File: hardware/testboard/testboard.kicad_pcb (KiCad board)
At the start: 2 copper layers, 175 x 140 mm, 22 parts, among them J1 Reset, P1 Conn_01x06, P2 Conn_01x06, U1 68LC040, U10 SN74ALVC164245, U11 ICE40HX4K-TQ144, U13 SST26VF023BA, U14 SN74ALVC164245, U15 SN74ALVC164245, U2 MAX232, U3 MAX232, U4 68681, U6 IS61C5128AS-25TLI, U7 IS61C5128AS-25TLI, U8 NB3N502, X1 ASE-33MHz, X2 33MHz, X3 33MHz

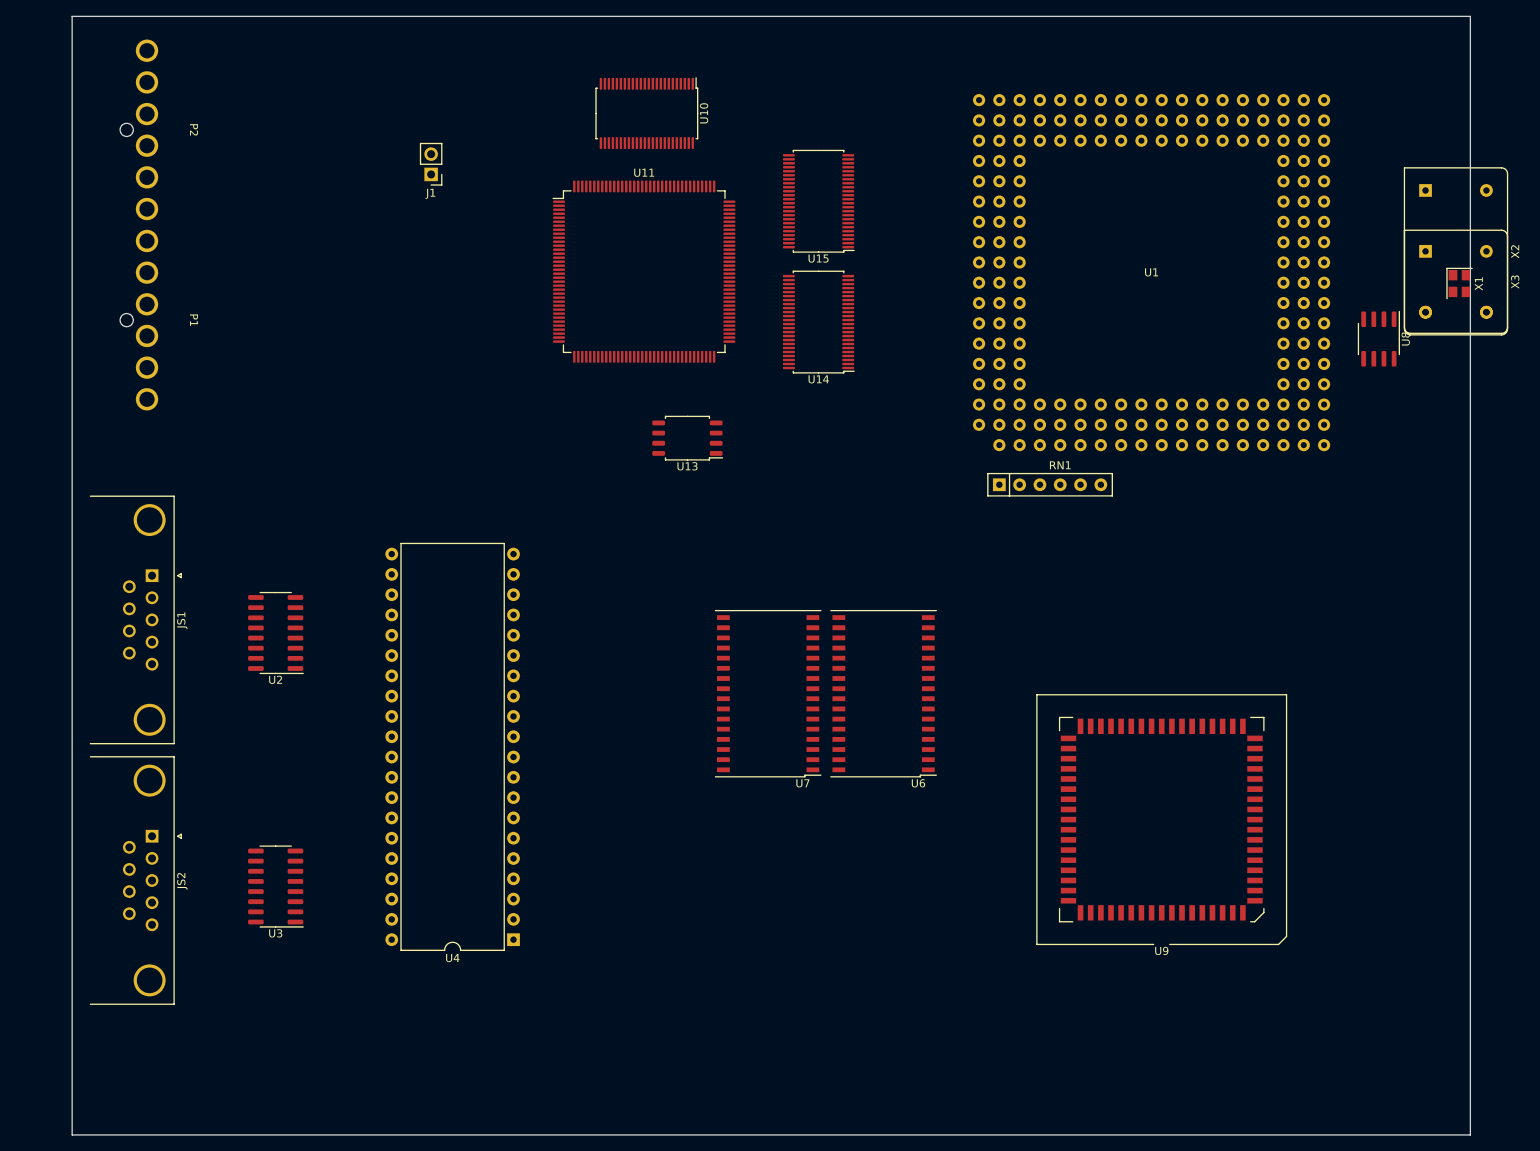
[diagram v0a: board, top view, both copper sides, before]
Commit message: simpleboard nearly complete
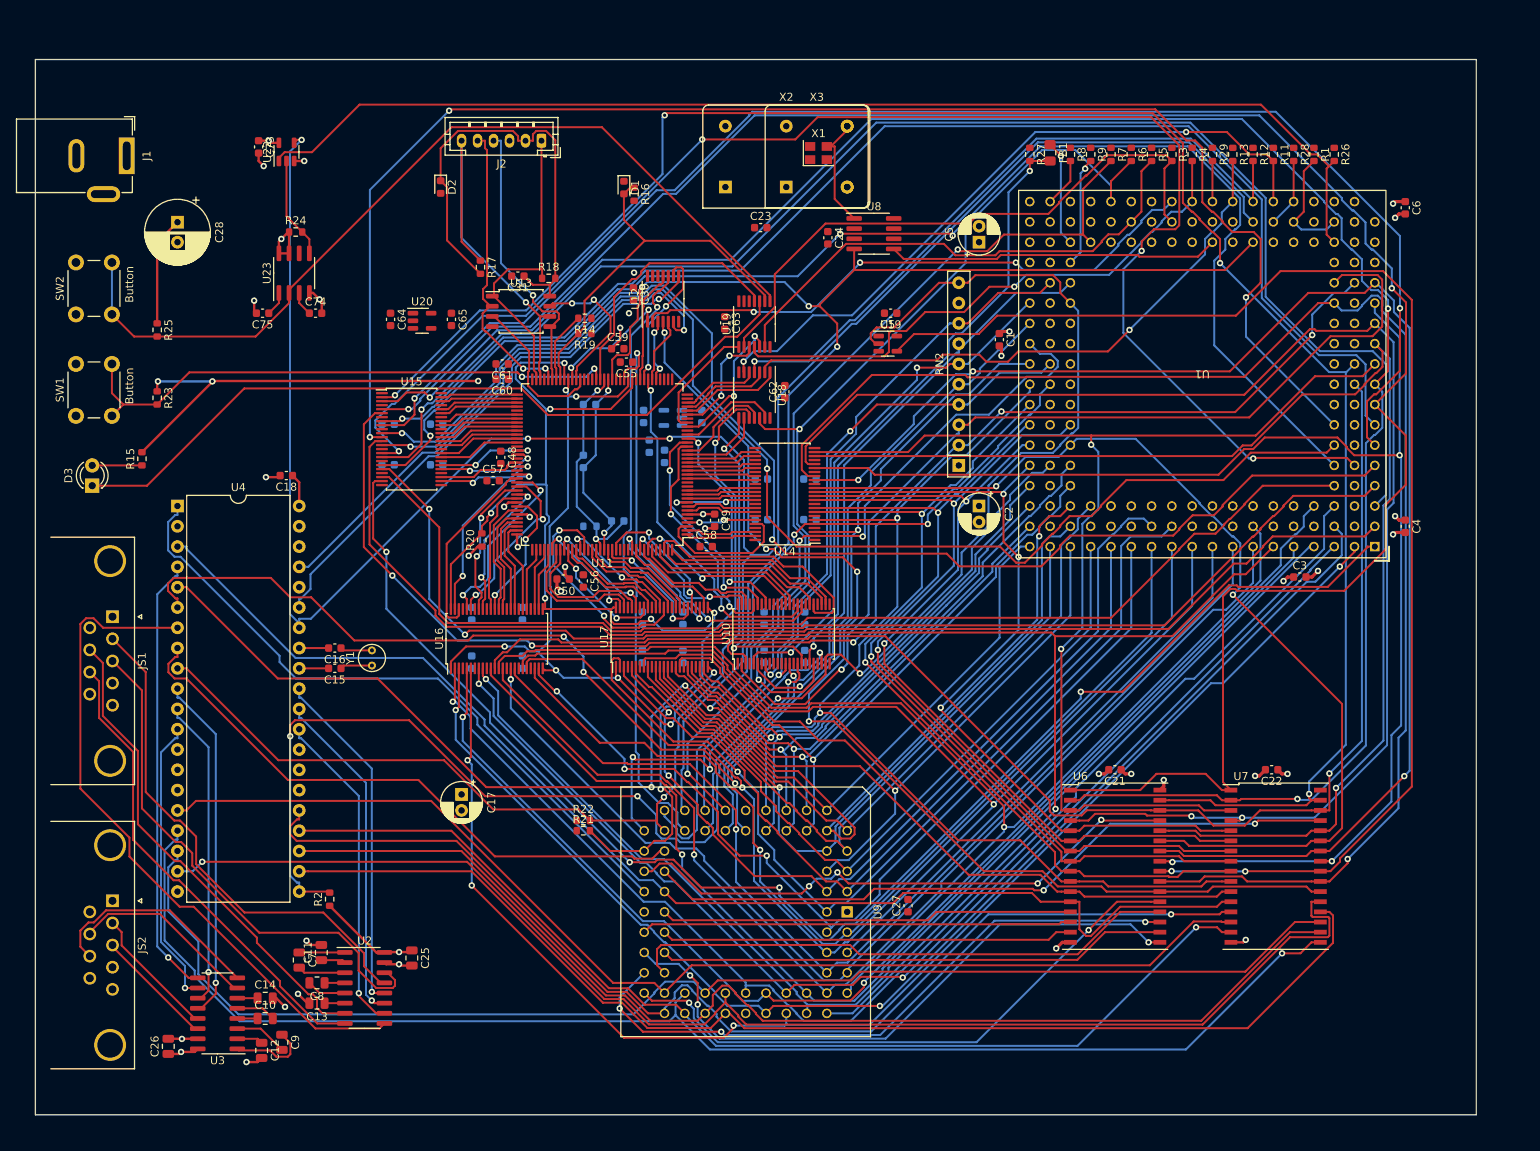
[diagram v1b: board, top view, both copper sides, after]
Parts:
- removed P1, P2: Conn_01x06, 68040:15-48-0106
- removed RN1: 4.7k, Resistor_THT:R_Array_SIP6
- added C1: 0.22uF, Capacitor_SMD:C_0603_1608Metric, F.Cu at (146.1, 60.5)
- added C10: 1uF, Capacitor_SMD:C_0805_2012Metric, F.Cu at (54.2, 145.4)
- added C11: 1uF, Capacitor_SMD:C_0805_2012Metric, F.Cu at (61.2, 137.2)
- added C12: 1uF, Capacitor_SMD:C_0805_2012Metric, F.Cu at (53.7, 149.4)
- added C13: 1uF, Capacitor_SMD:C_0805_2012Metric, F.Cu at (60.6, 143.5)
- added C14: 1uF, Capacitor_SMD:C_0805_2012Metric, F.Cu at (54.2, 142.9)
- added C15: 15pF, Capacitor_SMD:C_0603_1608Metric, F.Cu at (62.9, 101.6)
- added C16: 15pF, Capacitor_SMD:C_0603_1608Metric, F.Cu at (62.9, 99.1)
- added C17: C_Polarized_Small_US, Capacitor_THT:CP_Radial_D5.0mm_P2.00mm, F.Cu at (78.7, 117.4)
- added C18: 100nF, Capacitor_SMD:C_0603_1608Metric, F.Cu at (56.8, 77.5)
- added C19: 100nF, Capacitor_SMD:C_0603_1608Metric, F.Cu at (132.4, 57.1)
- added C2: 22uF, Capacitor_THT:CP_Radial_D5.0mm_P2.00mm, F.Cu at (143.5, 81.3)
- added C21: 100nF, Capacitor_SMD:C_0603_1608Metric, F.Cu at (160.5, 114.3)
- added C22: 100nF, Capacitor_SMD:C_0603_1608Metric, F.Cu at (180.1, 114.3)
- added C23: 100nF, Capacitor_SMD:C_0603_1608Metric, F.Cu at (116.2, 46.4)
- added C24: 100nF, Capacitor_SMD:C_0603_1608Metric, F.Cu at (124.6, 47.7)
- added C25: 1uF, Capacitor_SMD:C_0805_2012Metric, F.Cu at (72.5, 137.9)
- added C26: 1uF, Capacitor_SMD:C_0805_2012Metric, F.Cu at (42.0, 148.9)
- added C27: 100nF, Capacitor_SMD:C_0603_1608Metric, F.Cu at (134.6, 131.3)
- added C28: 220uF, Capacitor_THT:CP_Radial_D8.0mm_P2.50mm, F.Cu at (43.2, 45.8)
- added C3: 220pF, Capacitor_SMD:C_0603_1608Metric, F.Cu at (183.7, 90.2)
- added C30: 100nF, Capacitor_SMD:C_0603_1608Metric, F.Cu at (100.2, 54.8)
- added C31: 100nF, Capacitor_SMD:C_0603_1608Metric, F.Cu at (85.8, 52.5)
- added C32: 100nF, Capacitor_SMD:C_0603_1608Metric, B.Cu at (122.3, 83.0)
- added C33: 100nF, Capacitor_SMD:C_0603_1608Metric, B.Cu at (122.3, 77.9)
- added C34: 100nF, Capacitor_SMD:C_0603_1608Metric, B.Cu at (116.3, 83.0)
- added C35: 100nF, Capacitor_SMD:C_0603_1608Metric, B.Cu at (116.3, 77.9)
- added C36: 100nF, Capacitor_SMD:C_0603_1608Metric, B.Cu at (75.6, 71.0)
- added C37: 100nF, Capacitor_SMD:C_0603_1608Metric, B.Cu at (75.6, 76.1)
- added C38: 100nF, Capacitor_SMD:C_0603_1608Metric, B.Cu at (69.5, 76.1)
- added C39: 100nF, Capacitor_SMD:C_0603_1608Metric, B.Cu at (69.5, 71.0)
- added C4: 0.22uF, Capacitor_SMD:C_0603_1608Metric, F.Cu at (196.8, 83.8)
- added C40: 100nF, Capacitor_SMD:C_0603_1608Metric, B.Cu at (101.4, 100.1)
- added C41: 100nF, Capacitor_SMD:C_0603_1608Metric, B.Cu at (80.0, 94.8)
- added C42: 100nF, Capacitor_SMD:C_0603_1608Metric, B.Cu at (86.4, 94.8)
- added C43: 100nF, Capacitor_SMD:C_0603_1608Metric, B.Cu at (106.4, 100.1)
- added C44: 100nF, Capacitor_SMD:C_0603_1608Metric, B.Cu at (101.4, 95.3)
- added C45: 100nF, Capacitor_SMD:C_0603_1608Metric, B.Cu at (80.0, 100.8)
- added C46: 100nF, Capacitor_SMD:C_0603_1608Metric, B.Cu at (106.4, 95.3)
- added C47: 100nF, Capacitor_SMD:C_0603_1608Metric, B.Cu at (86.4, 100.8)
- added C48: 100nF, Capacitor_SMD:C_0603_1608Metric, F.Cu at (83.6, 75.2)
- added C49: 100nF, Capacitor_SMD:C_0603_1608Metric, F.Cu at (110.4, 83.1)
- added C5: 22uF, Capacitor_THT:CP_Radial_D5.0mm_P2.00mm, F.Cu at (143.5, 48.3)
- added C50: 100nF, Capacitor_SMD:C_0603_1608Metric, F.Cu at (91.5, 90.4)
- added C51: 100nF, Capacitor_SMD:C_0603_1608Metric, B.Cu at (116.6, 100.1)
- added C52: 100nF, Capacitor_SMD:C_0603_1608Metric, B.Cu at (121.7, 100.1)
- added C53: 100nF, Capacitor_SMD:C_0603_1608Metric, B.Cu at (121.7, 95.3)
- added C54: 100nF, Capacitor_SMD:C_0603_1608Metric, B.Cu at (116.6, 95.3)
- added C55: 100nF, Capacitor_SMD:C_0603_1608Metric, F.Cu at (99.4, 63.3)
- added C56: 4.7uF, Capacitor_SMD:C_0603_1608Metric, F.Cu at (94.0, 90.7)
- added C57: 4.7uF, Capacitor_SMD:C_0603_1608Metric, F.Cu at (82.7, 78.1)
- added C58: 4.7uF, Capacitor_SMD:C_0603_1608Metric, F.Cu at (109.4, 86.4)
- added C59: 4.7uF, Capacitor_SMD:C_0603_1608Metric, F.Cu at (98.3, 61.6)
- added C6: 220pF, Capacitor_SMD:C_0603_1608Metric, F.Cu at (196.8, 44.0)
- added C60: 4.7uF, Capacitor_SMD:C_0603_1608Metric, F.Cu at (83.8, 65.4)
- added C61: 100nF, Capacitor_SMD:C_0603_1608Metric, F.Cu at (83.8, 63.5)
- added C62: 100nF, Capacitor_SMD:C_0603_1608Metric, F.Cu at (119.2, 67.0)
- added C63: 100nF, Capacitor_SMD:C_0603_1608Metric, F.Cu at (111.7, 58.4)
- added C64: 4.7uF, Capacitor_SMD:C_0603_1608Metric, F.Cu at (69.8, 57.9)
- added C65: 4.7uF, Capacitor_SMD:C_0603_1608Metric, F.Cu at (77.5, 57.9)
- added C66: 4.7uF, Capacitor_SMD:C_0603_1608Metric, B.Cu at (108.8, 70.1)
- added C67: 4.7uF, Capacitor_SMD:C_0603_1608Metric, B.Cu at (101.5, 70.1)
- added C68: 100nF, Capacitor_SMD:C_0603_1608Metric, B.Cu at (102.2, 73.8)
- added C69: 4.7uF, Capacitor_SMD:C_0603_1608Metric, B.Cu at (104.1, 75.1)
- added C7: 1uF, Capacitor_SMD:C_0805_2012Metric, F.Cu at (58.4, 138.1)
- added C70: 100nF, Capacitor_SMD:C_0603_1608Metric, B.Cu at (94.8, 68.6)
- added C71: 100nF, Capacitor_SMD:C_0603_1608Metric, B.Cu at (98.3, 83.2)
- added C72: 4.7uF, Capacitor_SMD:C_0603_1608Metric, B.Cu at (94.0, 75.7)
- added C73: 100nF, Capacitor_SMD:C_0603_1608Metric, F.Cu at (53.3, 36.3)
- added C74: 100nF, Capacitor_SMD:C_0603_1608Metric, F.Cu at (60.5, 57.1)
- added C75: 100nF, Capacitor_SMD:C_0603_1608Metric, F.Cu at (53.8, 57.1)
- added C8: 1uF, Capacitor_SMD:C_0805_2012Metric, F.Cu at (60.6, 141.0)
- added C9: 1uF, Capacitor_SMD:C_0805_2012Metric, F.Cu at (56.3, 148.4)
- added D1: LTST-C191KGKT, LED_SMD:LED_0603_1608Metric, F.Cu at (99.1, 41.4)
- added D2: D_Schottky, Diode_SMD:D_0603_1608Metric, F.Cu at (76.1, 41.4)
- added D3: LED, LED_THT:LED_D3.0mm, F.Cu at (32.5, 78.7)
- added FB1: FerriteBead, Inductor_SMD:L_0805_2012Metric_Pad1.15x1.40mm_HandSolder, F.Cu at (152.4, 37.1)
- added J2: Conn_01x06, Connector_JST:JST_PH_B6B-PH-K_1x06_P2.00mm_Vertical, F.Cu at (88.7, 35.6)
- added R1: 4.7k, Resistor_SMD:R_0603_1608Metric, F.Cu at (185.4, 37.3)
- added R10: 100, Resistor_SMD:R_0603_1608Metric, B.Cu at (94.8, 83.8)
- added R11: 4.7k, Resistor_SMD:R_0603_1608Metric, F.Cu at (180.3, 37.3)
- added R12: 4.7k, Resistor_SMD:R_0603_1608Metric, F.Cu at (177.8, 37.3)
- added R13: 4.7k, Resistor_SMD:R_0603_1608Metric, F.Cu at (175.3, 37.3)
- added R14: 10k, Resistor_SMD:R_0603_1608Metric, F.Cu at (94.2, 57.8)
- added R15: 2.2K, Resistor_SMD:R_0603_1608Metric, F.Cu at (38.7, 75.4)
- added R16: 2.2K, Resistor_SMD:R_0603_1608Metric, F.Cu at (100.3, 42.3)
- added R17: 10K, Resistor_SMD:R_0603_1608Metric, F.Cu at (81.1, 51.4)
- added R18: 10K, Resistor_SMD:R_0603_1608Metric, F.Cu at (89.6, 52.8)
- added R19: 10k, Resistor_SMD:R_0603_1608Metric, F.Cu at (94.2, 59.7)
- added R2: 1k, Resistor_SMD:R_0603_1608Metric, F.Cu at (62.2, 130.5)
- added R20: R_Small_US, Resistor_SMD:R_0603_1608Metric, F.Cu at (81.3, 85.5)
- added R21: 1k, Resistor_SMD:R_0603_1608Metric, F.Cu at (94.0, 121.9)
- added R22: 1k, Resistor_SMD:R_0603_1608Metric, F.Cu at (94.0, 120.7)
- added R23: 1k, Resistor_SMD:R_0603_1608Metric, F.Cu at (40.6, 67.8)
- added R24: 1k, Resistor_SMD:R_0603_1608Metric, F.Cu at (58.0, 47.0)
- added R25: 1k, Resistor_SMD:R_0603_1608Metric, F.Cu at (40.6, 59.2)
- added R26: 4.7k, Resistor_SMD:R_0603_1608Metric, F.Cu at (188.0, 37.3)
- added R27: 4.7k, Resistor_SMD:R_0603_1608Metric, F.Cu at (149.9, 37.3)
- added R28: 4.7k, Resistor_SMD:R_0603_1608Metric, F.Cu at (182.9, 37.3)
- added R29: 4.7k, Resistor_SMD:R_0603_1608Metric, F.Cu at (172.7, 37.3)
- added R3: 4.7k, Resistor_SMD:R_0603_1608Metric, F.Cu at (167.6, 37.3)
- added R4: 4.7k, Resistor_SMD:R_0603_1608Metric, F.Cu at (170.2, 37.3)
- added R5: 4.7k, Resistor_SMD:R_0603_1608Metric, F.Cu at (165.1, 37.3)
- added R6: 4.7k, Resistor_SMD:R_0603_1608Metric, F.Cu at (162.6, 37.3)
- added R7: 4.7k, Resistor_SMD:R_0603_1608Metric, F.Cu at (160.0, 37.3)
- added R8: 4.7k, Resistor_SMD:R_0603_1608Metric, F.Cu at (154.9, 37.3)
- added R9: 4.7k, Resistor_SMD:R_0603_1608Metric, F.Cu at (157.5, 37.3)
- added RN2: 1k, Resistor_THT:R_Array_SIP10, F.Cu at (141.0, 76.2)
- added SW1: Button, Button_Switch_THT:SW_PUSH_6mm, F.Cu at (30.5, 70.0)
- added SW2: Button, Button_Switch_THT:SW_PUSH_6mm, F.Cu at (30.5, 57.3)
- added U12: 74AHCT04, Package_SO:TSSOP-14_4.4x5mm_P0.65mm, F.Cu at (104.0, 55.4)
- added U16: SN74ALVC164245, Package_SO:TSSOP-48_6.1x12.5mm_P0.5mm, F.Cu at (83.2, 97.9)
- added U17: SN74ALVC164245, Package_SO:TSSOP-48_6.1x12.5mm_P0.5mm, F.Cu at (103.8, 97.7)
- added U18: SN74LVC07, Package_SO:TSSOP-14_4.4x5mm_P0.65mm, F.Cu at (115.4, 67.4)
- added U19: SN74LVC07, Package_SO:TSSOP-14_4.4x5mm_P0.65mm, F.Cu at (115.4, 58.5)
- added U20: AP2112K-3.3, Package_TO_SOT_SMD:SOT-23-5, F.Cu at (73.8, 58.1)
- added U21: AP2112K-1.2, Package_TO_SOT_SMD:SOT-23-5, B.Cu at (105.2, 70.2)
- added U22: 74LVC1G08, Package_TO_SOT_SMD:SOT-23-5, F.Cu at (56.8, 37.0)
- added U23: TL7705A, Package_SO:SOIC-8_3.9x4.9mm_P1.27mm, F.Cu at (57.8, 52.1)
- added U5: 74LVC1G04, Package_TO_SOT_SMD:SOT-23-5, F.Cu at (132.1, 61.0)
- added Y1: 3.6864MHz, Crystal:Crystal_C38-LF_D3.0mm_L8.0mm_Vertical, F.Cu at (67.5, 101.2)
- J1: value Reset -> Barrel_Jack; footprint Connector_PinHeader_2.54mm:PinHeader_1x02_P2.54mm_Vertical -> Connector_BarrelJack:BarrelJack_GCT_DCJ200-10-A_Horizontal
- U9: footprint Package_LCC:PLCC-68_SMD-Socket -> Package_LCC:PLCC-68_THT-Socket
- moved X2 87.6 mm to (111.8, 41.4), turned to 0 degrees
- moved X1 81.9 mm to (123.4, 37.1), turned to 0 degrees
- moved X3 80.4 mm to (119.4, 41.4), turned to 0 degrees
- moved U1 74.7 mm to (193.0, 86.4), turned to 180 degrees
- moved U4 68.7 mm to (43.2, 81.3), turned to 0 degrees
- moved U10 67.4 mm to (119.0, 97.3), turned to 90 degrees
- moved U7 67.1 mm to (180.6, 126.4), turned to 0 degrees
- moved U8 64.6 mm to (130.3, 47.2), turned to 0 degrees
- moved U15 59.0 mm to (72.5, 72.9), turned to 0 degrees
- moved U2 45.8 mm to (66.6, 141.6), turned to 0 degrees
- moved U9 41.0 mm to (127.0, 132.1), turned to -90 degrees
- moved J1 38.2 mm to (36.8, 37.5), turned to -90 degrees
- moved U6 36.1 mm to (160.5, 126.4), turned to 0 degrees
- moved U13 26.2 mm to (86.2, 56.9), turned to 0 degrees
- moved U11 24.7 mm to (96.3, 76.1), turned to 180 degrees
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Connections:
- J1 pad 1: unconnected-(J1-Pin_1-Pad1) -> +5V
- U1 pad R16: /~{TS} -> Net-(U1A-~{TS})
- U1 pad R3: /CPU/~{SW_RST} -> /~{SW_RST}
- U1 pad S11: /~{TCI}/~{TBI} -> /~{TBI}
- U1 pad S7: /CPU/~{HW_RST} -> /~{RST}
- U1 pad T10: /~{TCI}/~{TBI} -> /~{TCI}
- U10 pad 1: /FPGA/FPGA_D_DIR -> GND
- U10 pad 11: /PD30 -> GND
- U10 pad 12: /PD31 -> GND
- U10 pad 13: /PA0 -> /SIZ0
- U10 pad 14: /PA1 -> /SIZ1
- U10 pad 16: unconnected-(U10A-2B3-Pad16) -> /~{COM_IRQ}
- U10 pad 17: unconnected-(U10A-2B4-Pad17) -> /~{RST}
- U10 pad 19: unconnected-(U10A-2B5-Pad19) -> /~{TS}
- U10 pad 2: /PD24 -> /TT0
- U10 pad 20: unconnected-(U10A-2B6-Pad20) -> /~{TIP}
- U10 pad 22: /FPGA/~{68150_DS} -> /~{DS}
- U10 pad 23: unconnected-(U10A-2B8-Pad23) -> /R/~{W}
- U10 pad 26: unconnected-(U10A-2A8-Pad26) -> /FPGA/LV_R/~{W}
- U10 pad 29: unconnected-(U10A-2A6-Pad29) -> /FPGA/LV_~{TIP}
- U10 pad 3: /PD25 -> /TT1
- U10 pad 30: unconnected-(U10A-2A5-Pad30) -> /FPGA/LV_~{TS}
- U10 pad 32: unconnected-(U10A-2A4-Pad32) -> /FPGA/LV_~{RST}
- U10 pad 33: unconnected-(U10A-2A3-Pad33) -> /FPGA/LV_~{COM_IRQ}
- U10 pad 35: /FPGA/LV_PA1 -> /FPGA/LV_SIZ1
- U10 pad 36: /FPGA/LV_PA0 -> /FPGA/LV_SIZ0
- U10 pad 37: /FPGA/FPGA_D7 -> unconnected-(U10A-1A8-Pad37)
- U10 pad 38: /FPGA/FPGA_D6 -> unconnected-(U10A-1A7-Pad38)
- U10 pad 40: /FPGA/FPGA_D5 -> unconnected-(U10A-1A6-Pad40)
- U10 pad 41: /FPGA/FPGA_D4 -> /FPGA/LV_TM2
- U10 pad 43: /FPGA/FPGA_D3 -> /FPGA/LV_TM1
- U10 pad 44: /FPGA/FPGA_D2 -> /FPGA/LV_TM0
- U10 pad 46: /FPGA/FPGA_D1 -> /FPGA/LV_TT1
- U10 pad 47: /FPGA/FPGA_D0 -> /FPGA/LV_TT0
- U10 pad 48: /FPGA/FPGA_D_~{OE} -> GND
- U10 pad 5: /PD26 -> /TM0
- U10 pad 6: /PD27 -> /TM1
- U10 pad 8: /PD28 -> /TM2
- U10 pad 9: /PD29 -> GND
- U11 pad 1: /FPGA/~{DSACK0} -> /FPGA/LV.A0
- U11 pad 10: unconnected-(U11D-IOL_5B-Pad10) -> /FPGA/LV.A7
- U11 pad 101: /FPGA/LV.A23 -> /FPGA/LV_D7
- U11 pad 102: /FPGA/LV.A24 -> /FPGA/LV_D8
- U11 pad 104: /FPGA/LV.A25 -> /FPGA/LV_D9
- U11 pad 105: /FPGA/LV.A26 -> /FPGA/LV_D10
- U11 pad 106: /FPGA/LV.A27 -> /FPGA/LV_D11
- U11 pad 107: /FPGA/LV.A28 -> /FPGA/LV_D12
- U11 pad 109: +3.3V -> unconnected-(U11E-VPP_FAST-Pad109)
- U11 pad 11: unconnected-(U11D-IOL_8A-Pad11) -> /FPGA/LV.A8
- U11 pad 110: /FPGA/LV.A29 -> /FPGA/LV_D13
- U11 pad 111: +3.3V -> +1V2
- U11 pad 112: /FPGA/LV.A30 -> /FPGA/LV_D14
- U11 pad 113: /FPGA/LV.A31 -> /FPGA/LV_D15
- U11 pad 114: /FPGA/FPGA_D0 -> /FPGA/LV_D16
- U11 pad 115: /FPGA/FPGA_D1 -> /FPGA/LV_D17
- U11 pad 116: /FPGA/FPGA_D2 -> /FPGA/LV_D18
- U11 pad 117: /FPGA/FPGA_D3 -> /FPGA/LV_D19
- U11 pad 118: /FPGA/FPGA_D4 -> /FPGA/LV_D20
- U11 pad 119: /FPGA/FPGA_D5 -> /FPGA/LV_D21
- U11 pad 12: unconnected-(U11D-IOL_8B-Pad12) -> /FPGA/LV.A9
- U11 pad 120: /FPGA/FPGA_D6 -> /FPGA/LV_D22
- U11 pad 121: /FPGA/FPGA_D7 -> /FPGA/LV_D23
- U11 pad 122: unconnected-(U11A-IOT_190-Pad122) -> /FPGA/LV_D24
- U11 pad 124: unconnected-(U11A-IOT_191-Pad124) -> /FPGA/LV_D25
- U11 pad 125: unconnected-(U11A-IOT_192-Pad125) -> /FPGA/LV_D26
- U11 pad 126: +3.3V -> /FPGA/VCC_PLL
- U11 pad 127: GND -> /FPGA/GND_PLL
- U11 pad 128: unconnected-(U11A-IOT_197_GBIN1-Pad128) -> /FPGA/LV_D27
- U11 pad 129: unconnected-(U11A-IOT_198_GBIN0-Pad129) -> /FPGA/LV_D28
- U11 pad 130: unconnected-(U11A-IOT_206-Pad130) -> /FPGA/LV_D29
- U11 pad 134: unconnected-(U11A-IOT_212-Pad134) -> /FPGA/LV_D30
- U11 pad 135: unconnected-(U11A-IOT_213-Pad135) -> /FPGA/LV_D31
- U11 pad 136: unconnected-(U11A-IOT_214-Pad136) -> /FPGA/LV_TT0
- U11 pad 137: unconnected-(U11A-IOT_215-Pad137) -> /FPGA/LV_TT1
- U11 pad 138: unconnected-(U11A-IOT_216-Pad138) -> /FPGA/LV_SIZ0
- U11 pad 139: unconnected-(U11A-IOT_217-Pad139) -> /FPGA/LV_SIZ1
- U11 pad 141: unconnected-(U11A-IOT_219-Pad141) -> /FPGA/LV_~{TS}
- U11 pad 142: unconnected-(U11A-IOT_220-Pad142) -> /FPGA/LV_~{TIP}
- U11 pad 143: unconnected-(U11A-IOT_221-Pad143) -> /FPGA/LV_~{68150_DS}
- U11 pad 144: unconnected-(U11A-IOT_222-Pad144) -> /FPGA/LV_R/~{W}
- U11 pad 15: unconnected-(U11D-IOL_10A-Pad15) -> /FPGA/LV.A10
- U11 pad 16: unconnected-(U11D-IOL_10B-Pad16) -> /FPGA/LV.A11
- U11 pad 17: unconnected-(U11D-IOL_12A-Pad17) -> /FPGA/LV.A12
- U11 pad 18: unconnected-(U11D-IOL_12B-Pad18) -> /FPGA/LV.A13
- U11 pad 19: unconnected-(U11D-IOL_13A-Pad19) -> /FPGA/LV.A14
- U11 pad 2: /FPGA/~{DSACK1} -> /FPGA/LV.A1
- U11 pad 20: unconnected-(U11D-IOL_13B_GBIN7-Pad20) -> /FPGA/LV.A15
- U11 pad 21: unconnected-(U11D-IOL_14A_GBIN6-Pad21) -> /FPGA/LV_~{DSACK0}
- U11 pad 22: unconnected-(U11D-IOL_14B-Pad22) -> /FPGA/LV_~{DSACK1}
- U11 pad 23: unconnected-(U11D-IOL_17A-Pad23) -> /FPGA/LV_TM0
- U11 pad 24: unconnected-(U11D-IOL_17B-Pad24) -> /FPGA/LV_TM1
- U11 pad 25: unconnected-(U11D-IOL_18A-Pad25) -> /FPGA/LV_TM2
- U11 pad 26: unconnected-(U11D-IOL_18B-Pad26) -> /FPGA/LV_~{TA}
- U11 pad 27: +3.3V -> +1V2
- U11 pad 28: unconnected-(U11D-IOL_23A-Pad28) -> /FPGA/LV_~{TEA}
- U11 pad 29: unconnected-(U11D-IOL_23B-Pad29) -> /FPGA/LV_~{TBI}
- U11 pad 3: unconnected-(U11D-IOL_3A-Pad3) -> /FPGA/LV.A2
- U11 pad 31: unconnected-(U11D-IOL_24A-Pad31) -> /FPGA/LV_~{TCI}
- U11 pad 32: unconnected-(U11D-IOL_24B-Pad32) -> /FPGA/LV_~{IPL0}
- U11 pad 33: unconnected-(U11D-IOL_25A-Pad33) -> /FPGA/LV_~{IPL1}
- U11 pad 34: unconnected-(U11D-IOL_25B-Pad34) -> /FPGA/LV_~{IPL2}
- U11 pad 4: unconnected-(U11D-IOL_3B-Pad4) -> /FPGA/LV.A3
- U11 pad 40: +3.3V -> +1V2
- U11 pad 41: unconnected-(U11C-IOB_63-Pad41) -> /FPGA/LV_RAM_CS
- U11 pad 42: unconnected-(U11C-IOB_64-Pad42) -> /FPGA/LV_COM_IACK
- U11 pad 43: unconnected-(U11C-IOB_71-Pad43) -> /FPGA/LV_~{COM_IRQ}
- U11 pad 44: unconnected-(U11C-IOB_72-Pad44) -> /FPGA/LV_COM_CS
- U11 pad 45: unconnected-(U11C-IOB_73-Pad45) -> /FPGA/LV_68150_CS
- U11 pad 47: unconnected-(U11C-IOB_79-Pad47) -> /FPGA/FPGA_D_~{OE}
- U11 pad 48: unconnected-(U11C-IOB_80-Pad48) -> /FPGA/FPGA_D_DIR
- U11 pad 49: unconnected-(U11C-IOB_81_GBIN5-Pad49) -> /FPGA/LV_~{RST}
- U11 pad 53: GND -> /FPGA/GND_PLL
- U11 pad 54: +3.3V -> /FPGA/VCC_PLL
- U11 pad 55: /FPGA/FPGA_A_DIR -> /FPGA/FPGA_LED
- U11 pad 56: /FPGA/FPGA_A_~{OE} -> /FPGA/FPGA_BTN
- U11 pad 66: unconnected-(U11E-~{CRESET}-Pad66) -> Net-(U11E-~{CRESET})
- U11 pad 7: unconnected-(U11D-IOL_4A-Pad7) -> /FPGA/LV.A4
- U11 pad 73: /FPGA/LV.A0 -> /FPGA/LV.A16
- U11 pad 74: /FPGA/LV.A1 -> /FPGA/LV.A17
- U11 pad 75: /FPGA/LV.A2 -> /FPGA/LV.A18
- U11 pad 76: /FPGA/LV.A3 -> /FPGA/LV.A19
- U11 pad 78: /FPGA/LV.A4 -> /FPGA/LV.A20
- U11 pad 79: /FPGA/LV.A5 -> /FPGA/LV.A21
- U11 pad 8: unconnected-(U11D-IOL_4B-Pad8) -> /FPGA/LV.A5
- U11 pad 80: /FPGA/LV.A6 -> /FPGA/LV.A22
- U11 pad 81: /FPGA/LV.A7 -> /FPGA/LV.A23
- U11 pad 82: /FPGA/LV.A8 -> /FPGA/LV.A24
- U11 pad 83: /FPGA/LV.A9 -> /FPGA/LV.A25
- U11 pad 84: /FPGA/LV.A10 -> /FPGA/LV.A26
- U11 pad 85: /FPGA/LV.A11 -> /FPGA/LV.A27
- U11 pad 87: /FPGA/LV.A12 -> /FPGA/LV.A28
- U11 pad 88: /FPGA/LV.A13 -> /FPGA/LV.A29
- U11 pad 9: unconnected-(U11D-IOL_5A-Pad9) -> /FPGA/LV.A6
- U11 pad 90: /FPGA/LV.A14 -> /FPGA/LV.A30
- U11 pad 91: /FPGA/LV.A15 -> /FPGA/LV.A31
- U11 pad 92: +3.3V -> +1V2
- U11 pad 93: /FPGA/LV.A16 -> /FPGA/LV_D0
- U11 pad 94: /FPGA/LV.A17 -> /FPGA/LV_D1
- U11 pad 95: /FPGA/LV.A18 -> /FPGA/LV_D2
- U11 pad 96: /FPGA/LV.A19 -> /FPGA/LV_D3
- U11 pad 97: /FPGA/LV.A20 -> /FPGA/LV_D4
- U11 pad 98: /FPGA/LV.A21 -> /FPGA/LV_D5
- U11 pad 99: /FPGA/LV.A22 -> /FPGA/LV_D6
- U14 pad 1: /FPGA/FPGA_A_DIR -> GND
- U14 pad 24: /FPGA/FPGA_A_DIR -> GND
- U14 pad 25: /FPGA/FPGA_A_~{OE} -> GND
- U14 pad 48: /FPGA/FPGA_A_~{OE} -> GND
- U15 pad 1: /FPGA/FPGA_A_DIR -> GND
- U15 pad 24: /FPGA/FPGA_A_DIR -> GND
- U15 pad 25: /FPGA/FPGA_A_~{OE} -> GND
- U15 pad 48: /FPGA/FPGA_A_~{OE} -> GND
- U4 pad 34: /IO/~{RESET} -> /~{RST}
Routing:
- net /~{RST}: track 0.00 -> 265.3 mm, vias 0 -> 4
- net /A18: track 0.00 -> 261.0 mm, vias 0 -> 2
- net /A17: track 0.00 -> 251.9 mm, vias 0 -> 3
- net /A16: track 0.00 -> 236.9 mm, vias 0 -> 4
- net /A2: track 0.00 -> 231.4 mm, vias 0 -> 5
- net /A3: track 0.00 -> 227.9 mm, vias 0 -> 5
- net /A19: track 0.00 -> 212.1 mm, vias 0 -> 3
- net /A26: track 0.00 -> 188.9 mm, vias 0 -> 4
- net /A23: track 0.00 -> 187.5 mm, vias 0 -> 3
- net /A11: track 0.00 -> 186.4 mm, vias 0 -> 1
- net /A27: track 0.00 -> 183.6 mm, vias 0 -> 1
- net /A31: track 0.00 -> 181.3 mm, vias 0 -> 4
- net /A13: track 0.00 -> 180.6 mm, vias 0 -> 2
- net /A10: track 0.00 -> 179.9 mm, vias 0 -> 3
- net /A21: track 0.00 -> 179.8 mm, vias 0 -> 2
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- added copper zone on In2.Cu, net +3.3V
- added copper zone on In2.Cu, net +5V
- added copper zone on In1.Cu, net GND
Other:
- board size 175 x 140 mm -> 180.3 x 132.1 mm
- copper layers 2 -> 4
